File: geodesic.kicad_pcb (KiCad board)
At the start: 2 copper layers, 100 x 100 mm, 17 parts, among them J1 Program, J2 Base, U1 ATtiny24A-MU

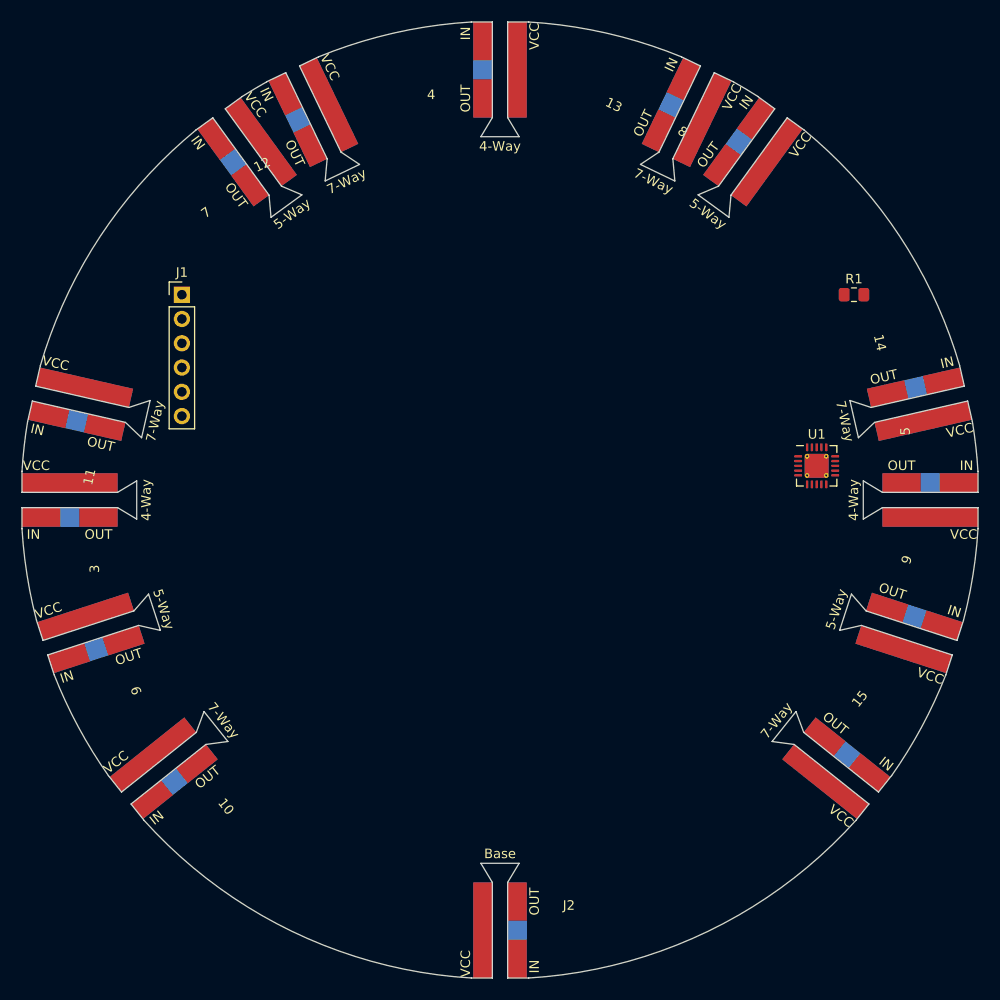
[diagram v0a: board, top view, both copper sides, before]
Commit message: Exported step files
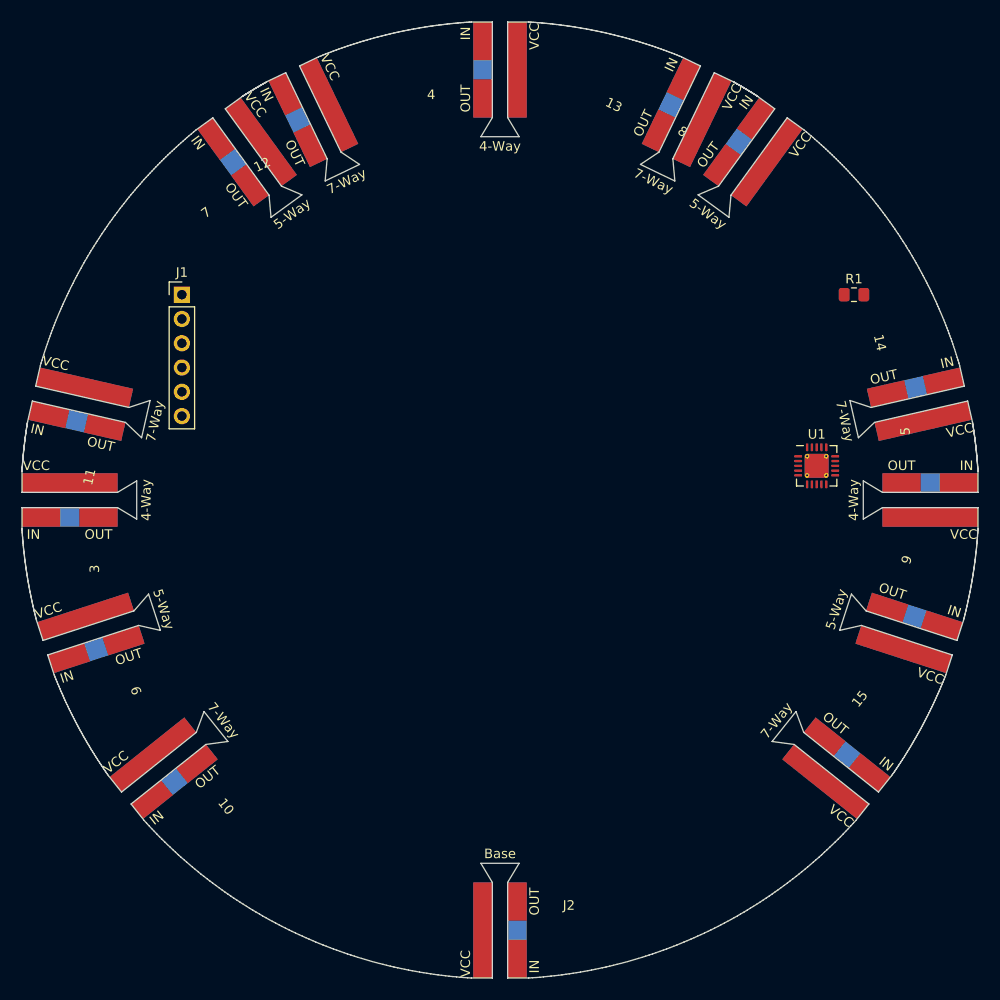
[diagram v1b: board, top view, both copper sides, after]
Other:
- outline, holes or cut-outs redrawn
